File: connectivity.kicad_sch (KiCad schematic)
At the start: 6 parts, among them J5 Conn_Coaxial, J6 Conn_Coaxial, U11 TCAN3404-Q1, U3 MAX-M10S, U4 MCP2518FD-xQBB, U9 Ai-Thinker-Ra-01H

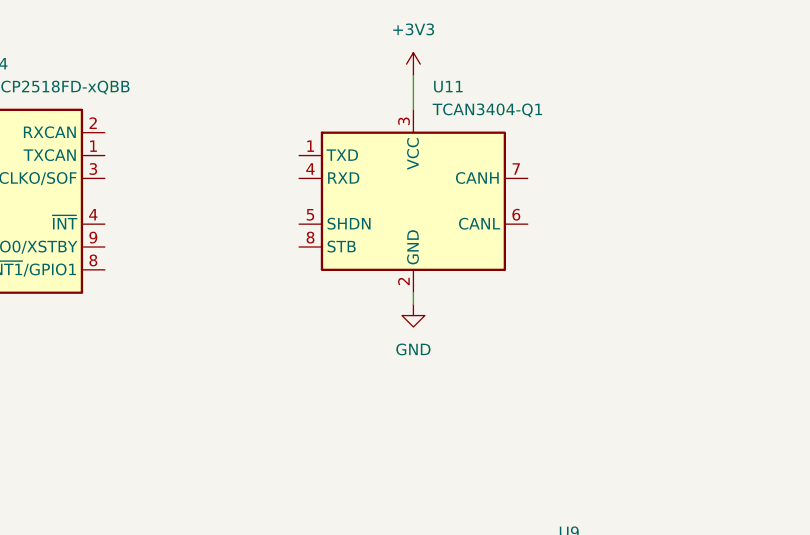
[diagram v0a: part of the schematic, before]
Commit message: Fixed BMI088 footprint and readme
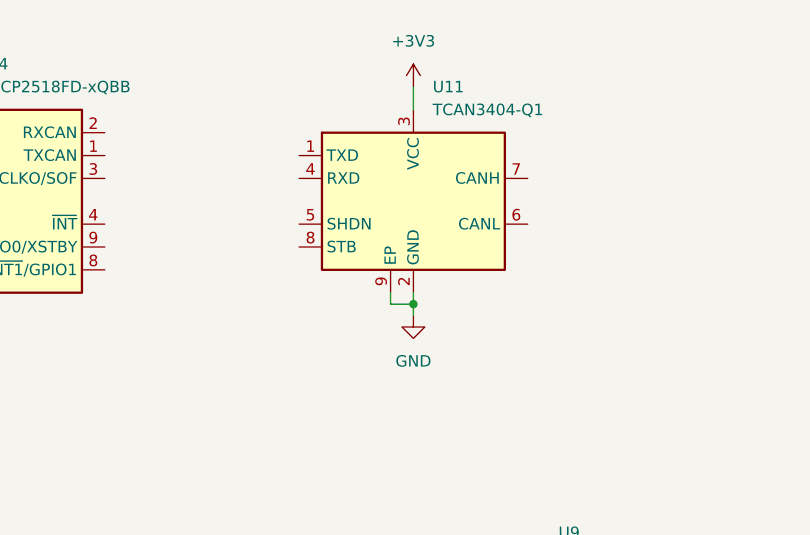
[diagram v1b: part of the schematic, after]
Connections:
- net GND: now also U11.9 (EP)
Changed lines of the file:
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@@
 	(generator_version "9.0")
 	(paper "A4")
+	(junction
+		(at 115.57 82.55)
+		(diameter 0)
+		(color 0 0 0 0)
+	)
+	(wire
+		(pts
+			(xy 113.03 82.55) (xy 115.57 82.55)
+		)
+		(stroke
+			(width 0)
+			(type default)
+		)
+	)
 	(wire
 		(pts
@@
 	(wire
 		(pts
-			(xy 115.57 57.15) (xy 115.57 60.96)
+			(xy 115.57 58.42) (xy 115.57 60.96)
 		)
 		(stroke
@@
 		(pts
 			(xy 115.57 81.28) (xy 115.57 82.55)
+		)
+		(stroke
+			(width 0)
+			(type default)
+		)
+	)
+	(wire
+		(pts
+			(xy 115.57 82.55) (xy 115.57 83.82)
+		)
+		(stroke
+			(width 0)
+			(type default)
+		)
+	)
+	(wire
+		(pts
+			(xy 113.03 81.28) (xy 113.03 82.55)
 		)
 		(stroke
@@
 	(symbol
 		(lib_id "power:GND")
-		(at 115.57 82.55 0)
+		(at 115.57 83.82 0)
 		(unit 1)
 		(exclude_from_sim no)
@@
 		(fields_autoplaced yes)
 		(property "Reference" "#PWR023"
+			(at 115.57 90.17 0)
+			(effects
+				(font
+					(size 1.27 1.27)
+				)
+				(hide yes)
+			)
+		)
+		(property "Value" "GND"
 			(at 115.57 88.9 0)
 			(effects
@@
 					(size 1.27 1.27)
 				)
-				(hide yes)
-			)
-		)
-		(property "Value" "GND"
-			(at 115.57 87.63 0)
-			(effects
-				(font
-					(size 1.27 1.27)
-				)
 			)
 		)
 		(property "Footprint" ""
-			(at 115.57 82.55 0)
+			(at 115.57 83.82 0)
 			(effects
 				(font
@@
 		)
 		(property "Datasheet" ""
-			(at 115.57 82.55 0)
+			(at 115.57 83.82 0)
 			(effects
 				(font
@@
 		)
 		(property "Description" "Power symbol creates a global label with name \"GND\" , ground"
-			(at 115.57 82.55 0)
+			(at 115.57 83.82 0)
 			(effects
 				(font
@@
 	(symbol
 		(lib_id "power:+3V3")
-		(at 115.57 57.15 0)
+		(at 115.57 58.42 0)
 		(unit 1)
 		(exclude_from_sim no)
@@
 		(fields_autoplaced yes)
 		(property "Reference" "#PWR024"
-			(at 115.57 60.96 0)
+			(at 115.57 62.23 0)
 			(effects
 				(font
@@
 		)
 		(property "Value" "+3V3"
-			(at 115.57 52.07 0)
+			(at 115.57 53.34 0)
 			(effects
 				(font
@@
 		)
 		(property "Footprint" ""
-			(at 115.57 57.15 0)
+			(at 115.57 58.42 0)
 			(effects
 				(font
@@
 		)
 		(property "Datasheet" ""
-			(at 115.57 57.15 0)
+			(at 115.57 58.42 0)
 			(effects
 				(font
@@
 		)
 		(property "Description" "Power symbol creates a global label with name \"+3V3\""
-			(at 115.57 57.15 0)
+			(at 115.57 58.42 0)
 			(effects
 				(font
@@
 		(pin "3"
 		)
-		(instances
+		(pin "9"
+		)
+		(instances
